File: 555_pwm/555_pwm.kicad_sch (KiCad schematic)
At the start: 5 parts, among them U1 NE555D

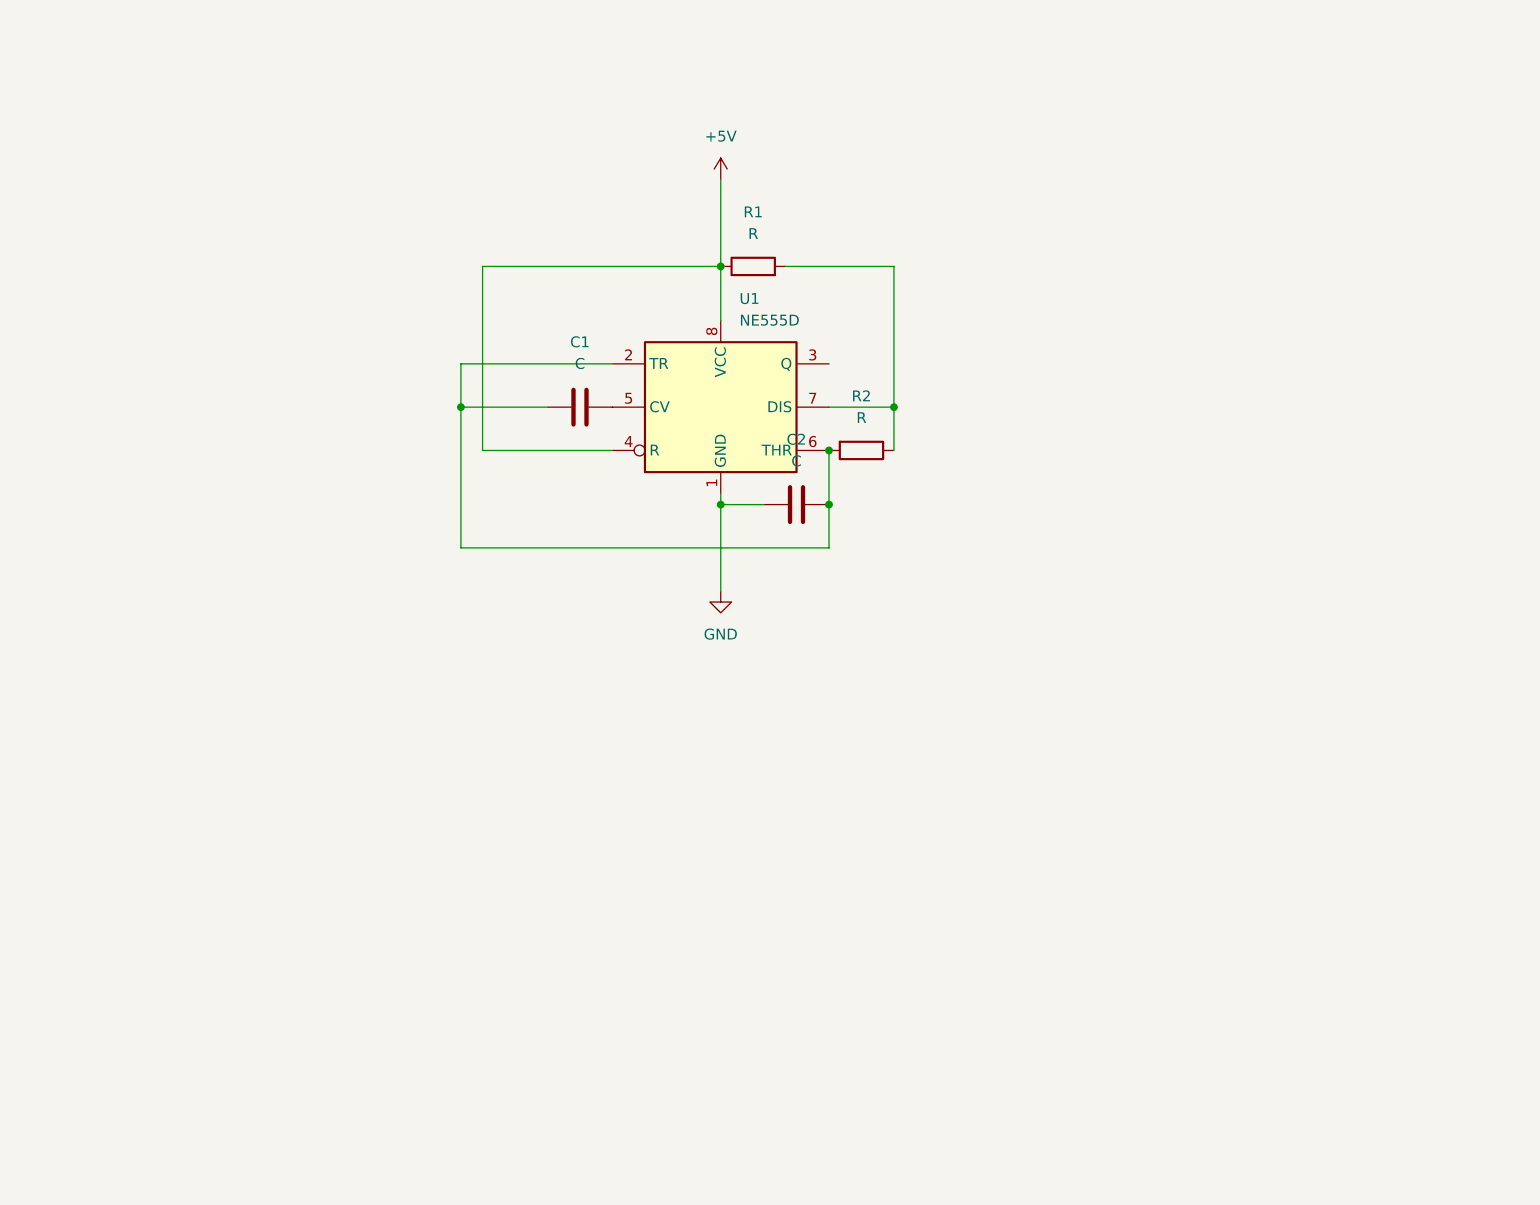
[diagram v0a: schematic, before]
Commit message: a
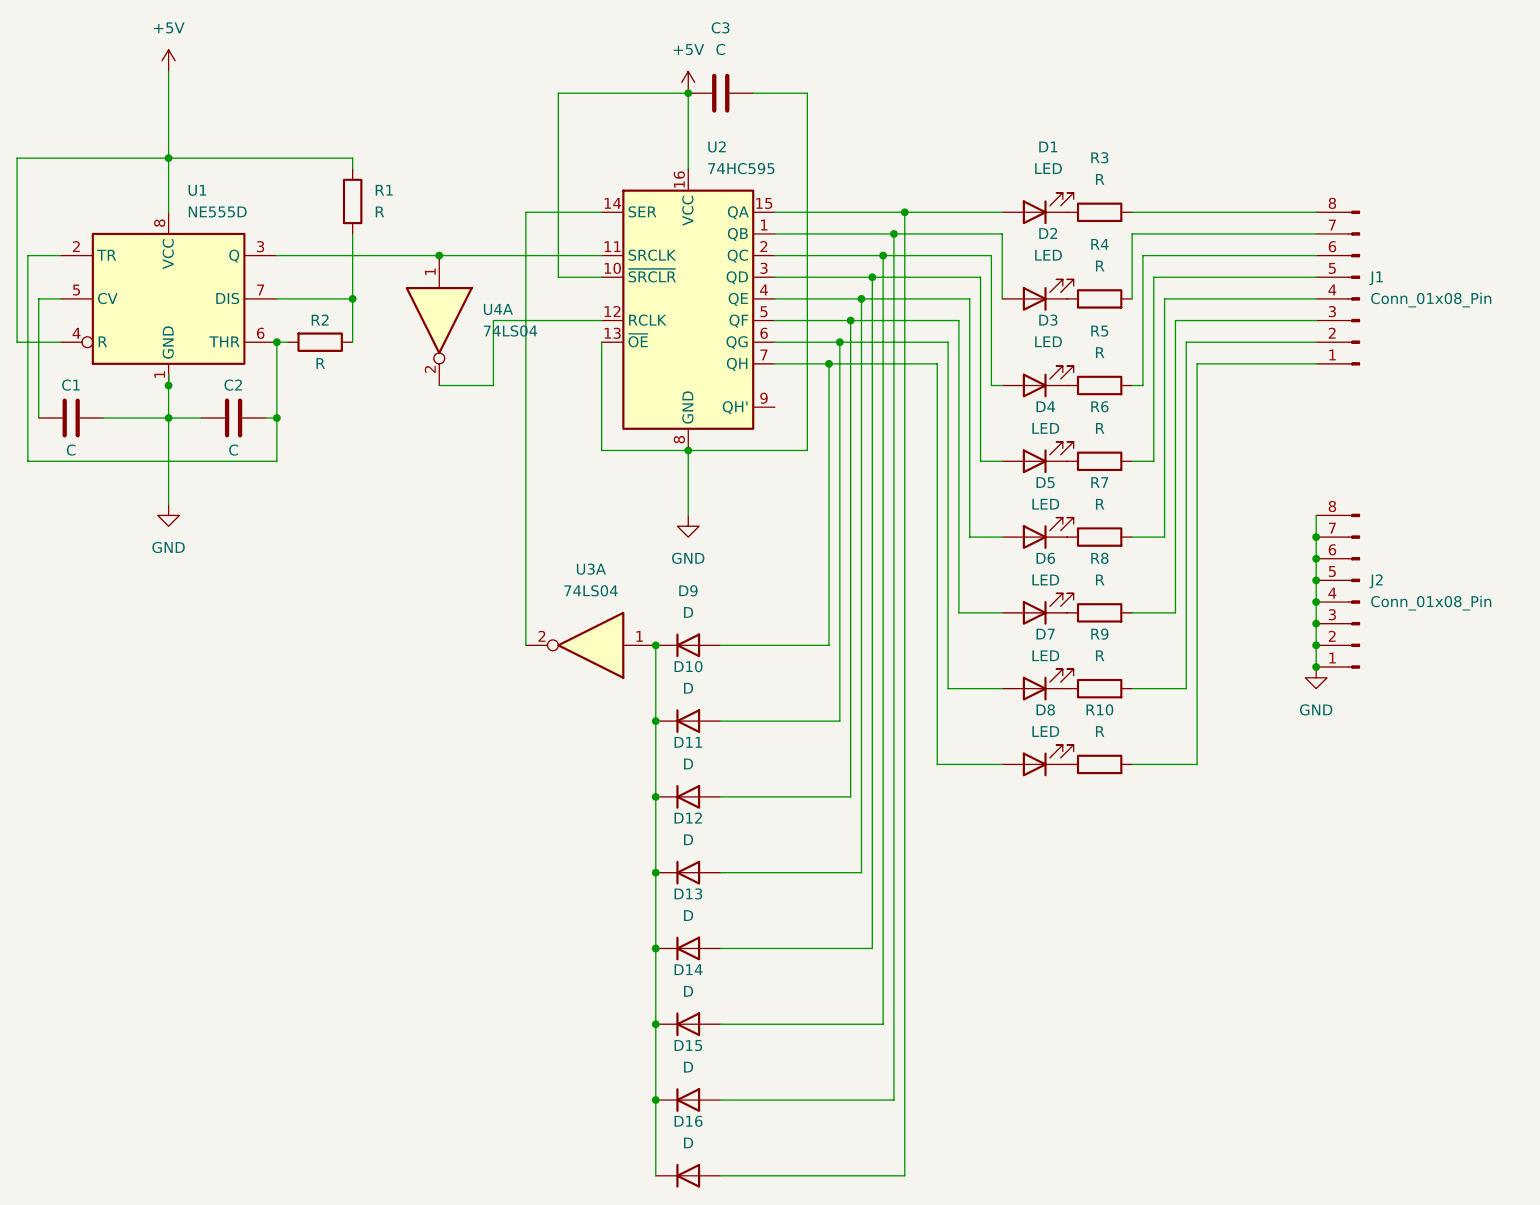
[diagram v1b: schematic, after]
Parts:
- added C3: C, symbol Device:C
- added D1, D2, D3, D4, D5, D6, D7, D8: LED, symbol Device:LED
- added D10, D11, D12, D13, D14, D15, D16, D9: D, symbol Device:D
- added J1, J2: Conn_01x08_Pin, symbol Connector:Conn_01x08_Pin
- added R10, R3, R4, R5, R6, R7, R8, R9: R, symbol Device:R
- added U2: 74HC595, symbol 74xx:74HC595
- added U3, U4: 74LS04, symbol 74xx:74LS04
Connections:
- net +5V: now also C3.1, U2.10 (~{SRCLR}), U2.16 (VCC)
- net GND: now also C1.1, C3.2, J2.1 (Pin_1), J2.2 (Pin_2), J2.3 (Pin_3), J2.4 (Pin_4), J2.5 (Pin_5), J2.6 (Pin_6), J2.7 (Pin_7), J2.8 (Pin_8), U2.13 (~{OE}), U2.8 (GND)
- net at C2.2, R2.2, U1.2 (TR)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: no longer C1.1
- net at U1.3 (Q): now also U2.11 (SRCLK), U4.1
- new net: D4.1 (K), R6.1
- new net: J1.5 (Pin_5), R6.2
- new net: D8.1 (K), R10.1
- new net: D8.2 (A), D9.2 (A), U2.7 (QH)
- new net: D10.1 (K), D11.1 (K), D12.1 (K), D13.1 (K), D14.1 (K), D15.1 (K), D16.1 (K), D9.1 (K), U3.1
- new net: U2.14 (SER), U3.2
- new net: D1.1 (K), R3.1
- new net: D1.2 (A), D16.2 (A), U2.15 (QA)
- new net: D3.1 (K), R5.1
- new net: D14.2 (A), D3.2 (A), U2.2 (QC)
- new net: D2.1 (K), R4.1
- new net: J1.7 (Pin_7), R4.2
- new net: D5.1 (K), R7.1
- new net: J1.4 (Pin_4), R7.2
- new net: D13.2 (A), D4.2 (A), U2.3 (QD)
- new net: D15.2 (A), D2.2 (A), U2.1 (QB)
- new net: D12.2 (A), D5.2 (A), U2.4 (QE)
- new net: J1.1 (Pin_1), R10.2
- new net: J1.2 (Pin_2), R9.2
- new net: J1.3 (Pin_3), R8.2
- new net: J1.6 (Pin_6), R5.2
- new net: J1.8 (Pin_8), R3.2
- new net: U2.12 (RCLK), U4.2
- new net: D10.2 (A), D7.2 (A), U2.6 (QG)
- new net: D7.1 (K), R9.1
- new net: D11.2 (A), D6.2 (A), U2.5 (QF)
- new net: D6.1 (K), R8.1
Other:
- moved on the sheet: C1, C2, R1, R2, U1
